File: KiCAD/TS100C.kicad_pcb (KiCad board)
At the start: 4 copper layers, 84 x 10 mm, 63 parts, among them J1 USB_C_Receptacle_USB2.0, J2 OLED_64x32, J3 A, J4 B, J5 DNP, P1 TC2030-CTX, Q1 SS8050, Q2 DMP3017SFG, SW1 key1, SW2 key2, U1 USBLC6-4SC6, U2 AP2204R-3.3, U3 STUSB4500, U4 STM32F072CBUx, U5 OPA340NA, U6 MCP9700AT-ETT, U7 SI8540

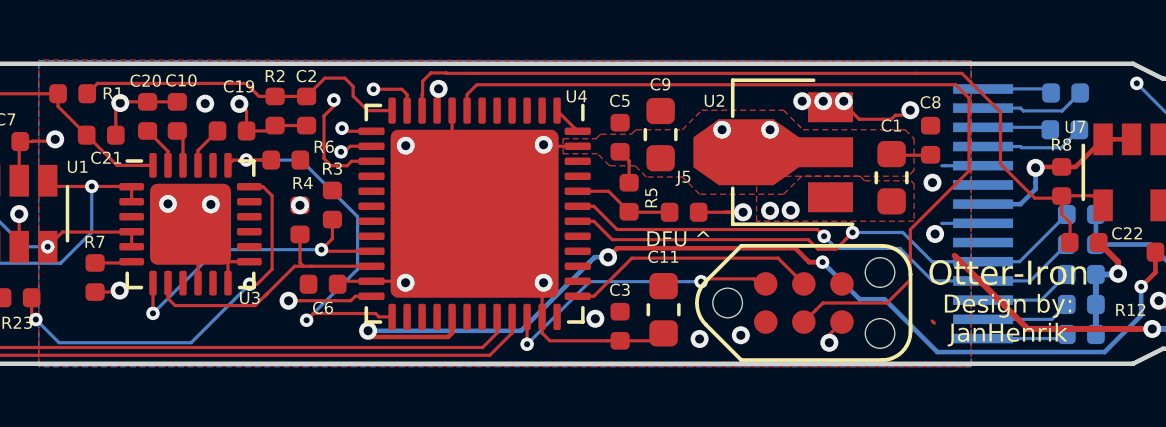
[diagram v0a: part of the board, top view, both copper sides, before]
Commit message: production files
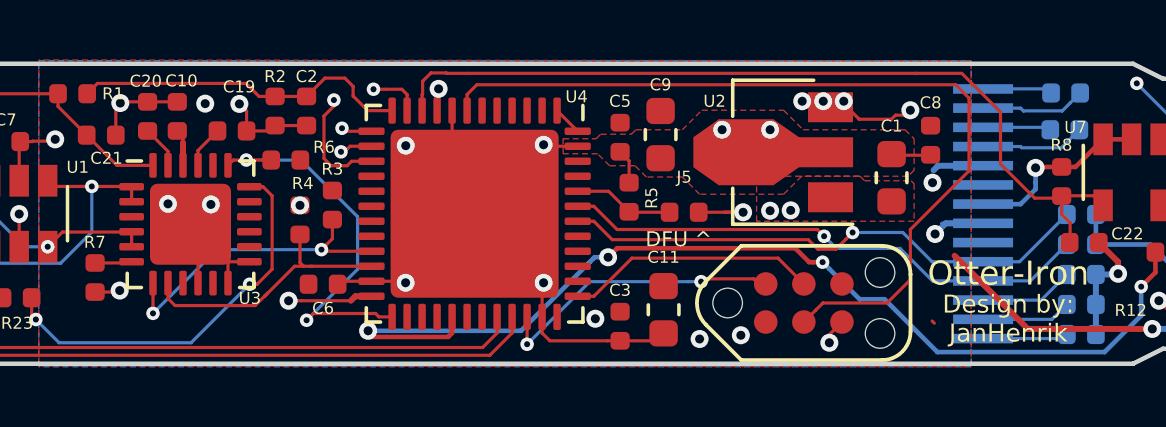
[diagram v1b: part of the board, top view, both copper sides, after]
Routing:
- net +3V3: track 73.7 -> 77.1 mm
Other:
- rule pad_to_mask_clearance: 0.1 -> 0
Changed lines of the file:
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@@
     (thickness 1.6)
     (drawings 12)
-    (tracks 626)
+    (tracks 631)
     (zones 0)
     (modules 63)
@@
   )
   (setup
-    (last_trace_width 0.154)
+    (last_trace_width 0.2)
     (user_trace_width 0.106)
     (user_trace_width 0.154)
@@
     (pad_size 1.71 2.37)
     (pad_drill 0)
-    (pad_to_mask_clearance 0.1)
-    (solder_mask_min_width 0.154)
+    (pad_to_mask_clearance 0)
     (aux_axis_origin 0 0)
     (visible_elements FFFFFF7F)
@@
       (drillshape 0)
       (scaleselection 1)
-      (outputdirectory "gerber/"))
+      (outputdirectory "gerber_2.3_fixed/"))
   )
   (net 0 "")
@@
   (segment (start 155.85 86.396) (end 155.85 82.925) (width 0.2) (layer B.Cu) (net 9))
   (segment (start 155.85 87.075) (end 155.85 86.396) (width 0.2) (layer B.Cu) (net 9))
-  (segment (start 106.8 81.5625) (end 106.8 80.887052) (width 0.106) (layer F.Cu) (net 9))
   (via (at 106.85 80.837052) (size 0.6) (drill 0.3) (layers F.Cu B.Cu) (net 9))
-  (segment (start 106.8 80.887052) (end 106.85 80.837052) (width 0.106) (layer F.Cu) (net 9))
   (segment (start 154.55 89) (end 142.35 89) (width 0.2) (layer B.Cu) (net 9))
   (segment (start 142.35 89) (end 142.25 88.9) (width 0.2) (layer B.Cu) (net 9))
@@
   (via (at 99.07 81.33) (size 0.6) (drill 0.3) (layers F.Cu B.Cu) (net 9))
   (segment (start 98.33 82.43) (end 98.14 82.24) (width 0.106) (layer F.Cu) (net 9))
-  (segment (start 98.33 83.3875) (end 98.33 82.43) (width 0.106) (layer F.Cu) (net 9))
   (via (at 122.575 81.55) (size 0.6) (drill 0.3) (layers F.Cu B.Cu) (net 9))
   (segment (start 140.3 85.325) (end 140.3 85.17401) (width 0.2) (layer F.Cu) (net 9))
@@
   (segment (start 115.52 84.95) (end 117 84.95) (width 0.106) (layer F.Cu) (net 9))
   (via (at 101.849996 87.9) (size 0.6) (drill 0.3) (layers F.Cu B.Cu) (net 9))
-  (segment (start 104.6125 87.75) (end 104.075 87.75) (width 0.106) (layer F.Cu) (net 9))
-  (segment (start 104.075 87.75) (end 103.925 87.9) (width 0.106) (layer F.Cu) (net 9))
   (segment (start 102.27426 87.9) (end 101.849996 87.9) (width 0.106) (layer F.Cu) (net 9))
   (segment (start 103.925 87.9) (end 102.27426 87.9) (width 0.106) (layer F.Cu) (net 9))
@@
   (segment (start 142.2625 87.2375) (end 142.1 87.075) (width 0.2) (layer B.Cu) (net 9))
   (segment (start 142.2625 88.9) (end 142.2625 87.2375) (width 0.2) (layer B.Cu) (net 9))
+  (segment (start 123.755 85.32) (end 123.4 85.675) (width 0.2) (layer B.Cu) (net 9))
+  (segment (start 125 85.32) (end 123.755 85.32) (width 0.2) (layer B.Cu) (net 9))
+  (segment (start 125 83.4) (end 123.5 83.4) (width 0.2) (layer B.Cu) (net 9))
+  (segment (start 123.5 83.4) (end 123.35 83.55) (width 0.2) (layer B.Cu) (net 9))
+  (segment (start 98.33 83.3875) (end 98.33 82.63) (width 0.2) (layer F.Cu) (net 9))
+  (segment (start 98.33 82.63) (end 98.33 82.43) (width 0.106) (layer F.Cu) (net 9))
+  (segment (start 106.8 80.887052) (end 106.85 80.837052) (width 0.2) (layer F.Cu) (net 9))
+  (segment (start 106.8 81.5625) (end 106.8 80.887052) (width 0.2) (layer F.Cu) (net 9))
+  (segment (start 104.075 87.75) (end 103.925 87.9) (width 0.2) (layer F.Cu) (net 9))
+  (segment (start 104.6125 87.75) (end 104.075 87.75) (width 0.2) (layer F.Cu) (net 9))
   (segment (start 97.83 87.3125) (end 97.83 87.825) (width 0.106) (layer F.Cu) (net 10))
   (segment (start 97.83 87.825) (end 98.065 88.06) (width 0.106) (layer F.Cu) (net 10))
@@
       )
     )
+  )
+  (zone (net 0) (net_name "") (layer B.Cu) (hatch edge 0.508)
+    (connect_pads (clearance 0.154))
+    (min_thickness 0.254)
+    (keepout (tracks allowed) (vias allowed) (copperpour not_allowed))
+    (fill (arc_segments 32) (thermal_gap 0.508) (thermal_bridge_width 0.508))
+    (polygon
+      (pts
+        (xy 123.85 80.5) (xy 126.15 80.5) (xy 126.15 89.5) (xy 123.85 89.5)
+      )
+    )
+  )
+  (zone (net 0) (net_name "") (layer F.Cu) (hatch edge 0.508)
+    (connect_pads (clearance 0.154))
+    (min_thickness 0.254)
+    (keepout (tracks allowed) (vias allowed) (copperpour not_allowed))
+    (fill (arc_segments 32) (thermal_gap 0.508) (thermal_bridge_width 0.508))
+    (polygon
+      (pts
+        (xy 98.1 82.9) (xy 98.55 82.9) (xy 98.55 83.8) (xy 98.1 83.8)
+      )
+    )
+  )
+  (zone (net 0) (net_name "") (layer F.Cu) (hatch edge 0.508)
+    (connect_pads (clearance 0.154))
+    (min_thickness 0.254)
+    (keepout (tracks allowed) (vias allowed) (copperpour not_allowed))
+    (fill (arc_segments 32) (thermal_gap 0.508) (thermal_bridge_width 0.508))
+    (polygon
+      (pts
+        (xy 106.55 80.95) (xy 107 80.95) (xy 107 82) (xy 106.55 82)
+      )
+    )
+  )
+  (zone (net 0) (net_name "") (layer F.Cu) (hatch edge 0.508)
+    (connect_pads (clearance 0.154))
+    (min_thickness 0.254)
+    (keepout (tracks allowed) (vias allowed) (copperpour not_allowed))
+    (fill (arc_segments 32) (thermal_gap 0.508) (thermal_bridge_width 0.508))
+    (polygon
+      (pts
+        (xy 104 87.5) (xy 105.1 87.5) (xy 105.1 88.05) (xy 104 88.05)
+      )
+    )
+  )
+  (zone (net 0) (net_name "") (layer F.Cu) (hatch edge 0.508)
+    (connect_pads (clearance 0.154))
+    (min_thickness 0.254)
+    (keepout (tracks allowed) (vias allowed) (copperpour not_allowed))
+    (fill (arc_segments 32) (thermal_gap 0.508) (thermal_bridge_width 0.508))
+    (polygon
+      (pts
+        (xy 110.95 88.05) (xy 110.7 88.05) (xy 110.7 89) (xy 110.55 89) (xy 110.55 87.95)
+        (xy 110.95 87.95)
+      )
+    )
+  )
+  (zone (net 0) (net_name "") (layer F.Cu) (hatch edge 0.508)
+    (connect_pads (clearance 0.154))
+    (min_thickness 0.254)
+    (keepout (tracks allowed) (vias allowed) (copperpour not_allowed))
+    (fill (arc_segments 32) (thermal_gap 0.508) (thermal_bridge_width 0.508))
+    (polygon
+      (pts
+        (xy 111.05 82.4) (xy 111.05 82) (xy 110.7 82) (xy 110.7 80.95) (xy 110.6 80.95)
+        (xy 110.6 82.1) (xy 110.95 82.1) (xy 110.95 82.4)
+      )
+    )
